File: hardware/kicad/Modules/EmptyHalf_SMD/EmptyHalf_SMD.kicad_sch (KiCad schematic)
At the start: 2 parts, among them J1 Conn_02x07_Odd_Even

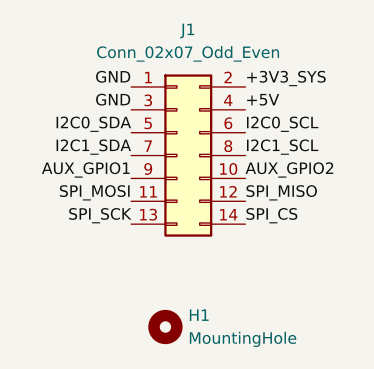
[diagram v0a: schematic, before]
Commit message: Add EEPROM slot address pin to module interface
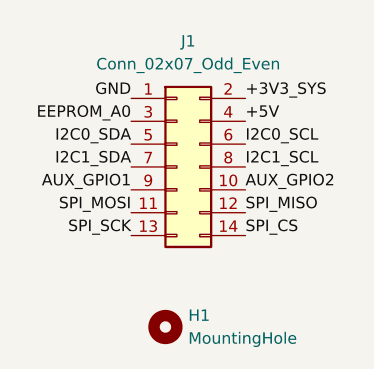
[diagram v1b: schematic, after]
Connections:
- net GND: no longer J1.3 (Pin_3)
- new net EEPROM_A0: J1.3 (Pin_3)
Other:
- moved on the sheet: J1
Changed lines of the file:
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@@
 	(paper "A4")
 	(label "SPI_MOSI"
-		(at 119.38 81.28 180)
+		(at 119.38 82.55 180)
 		(effects
 			(font
@@
 	)
 	(label "GND"
-		(at 119.38 68.58 180)
+		(at 119.38 69.85 180)
 		(effects
 			(font
@@
 	)
 	(label "I2C0_SDA"
-		(at 119.38 73.66 180)
+		(at 119.38 74.93 180)
 		(effects
 			(font
@@
 	)
 	(label "SPI_SCK"
-		(at 119.38 83.82 180)
+		(at 119.38 85.09 180)
 		(effects
 			(font
@@
 	)
 	(label "AUX_GPIO1"
-		(at 119.38 78.74 180)
+		(at 119.38 80.01 180)
 		(effects
 			(font
@@
 	)
 	(label "I2C0_SCL"
-		(at 132.08 73.66 0)
+		(at 132.08 74.93 0)
 		(effects
 			(font
@@
 	)
 	(label "I2C1_SDA"
-		(at 119.38 76.2 180)
+		(at 119.38 77.47 180)
 		(effects
 			(font
@@
 	)
 	(label "+3V3_SYS"
-		(at 132.08 68.58 0)
+		(at 132.08 69.85 0)
 		(effects
 			(font
@@
 	)
 	(label "I2C1_SCL"
-		(at 132.08 76.2 0)
+		(at 132.08 77.47 0)
 		(effects
 			(font
@@
 	)
 	(label "AUX_GPIO2"
-		(at 132.08 78.74 0)
+		(at 132.08 80.01 0)
 		(effects
 			(font
@@
 	)
 	(label "SPI_CS"
-		(at 132.08 83.82 0)
+		(at 132.08 85.09 0)
 		(effects
 			(font
@@
 	)
 	(label "+5V"
-		(at 132.08 71.12 0)
+		(at 132.08 72.39 0)
 		(effects
 			(font
@@
 		)
 	)
-	(label "GND"
-		(at 119.38 71.12 180)
+	(label "EEPROM_A0"
+		(at 119.38 72.39 180)
 		(effects
 			(font
@@
 	)
 	(label "SPI_MISO"
-		(at 132.08 81.28 0)
+		(at 132.08 82.55 0)
 		(effects
 			(font
@@
 	(symbol
 		(lib_id "Connector_Generic:Conn_02x07_Odd_Even")
-		(at 124.46 76.2 0)
+		(at 124.46 77.47 0)
 		(unit 1)
 		(body_style 1)
@@
 		(fields_autoplaced yes)
 		(property "Reference" "J1"
-			(at 125.73 62.23 0)
+			(at 125.73 63.5 0)
 			(show_name no)
 			(do_not_autoplace no)
@@
 		)
 		(property "Value" "Conn_02x07_Odd_Even"
-			(at 125.73 64.77 0)
+			(at 125.73 66.04 0)
 			(show_name no)
 			(do_not_autoplace no)
@@
 		)
 		(property "Footprint" "EnvNode-Footprints:J_Wurth_WR-PHD_61031421121"
-			(at 124.46 76.2 0)
+			(at 124.46 77.47 0)
 			(hide yes)
 			(show_name no)
@@
 		)
 		(property "Datasheet" ""
-			(at 124.46 76.2 0)
+			(at 124.46 77.47 0)
 			(hide yes)
 			(show_name no)
@@
 		)
 		(property "Description" "Generic connector, double row, 02x07, odd/even pin numbering scheme (row 1 odd numbers, row 2 even numbers), script generated (kicad-library-utils/schlib/autogen/connector/)"
-			(at 124.46 76.2 0)
+			(at 124.46 77.47 0)
 			(hide yes)
 			(show_name no)
